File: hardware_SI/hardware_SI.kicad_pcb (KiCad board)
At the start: 2 copper layers, 141.2 x 96.5 mm, 58 parts, among them J1 Barrel_Jack_Switch, J2 Conn_01x07_Female, J3 USB_B_Micro, Q1 SI2323DS-T1, Q2 SI2323DS-T1, SW1 SW_SPDT, U1 OMEGA2+, U2 LTC4085EDEPBF, U3 TPS61200DRC, U4 LD1117S33TR_SOT223, U5 MAX6369, U6 MCP3021, U7 USBLC6-2SC6, U8 CH340N

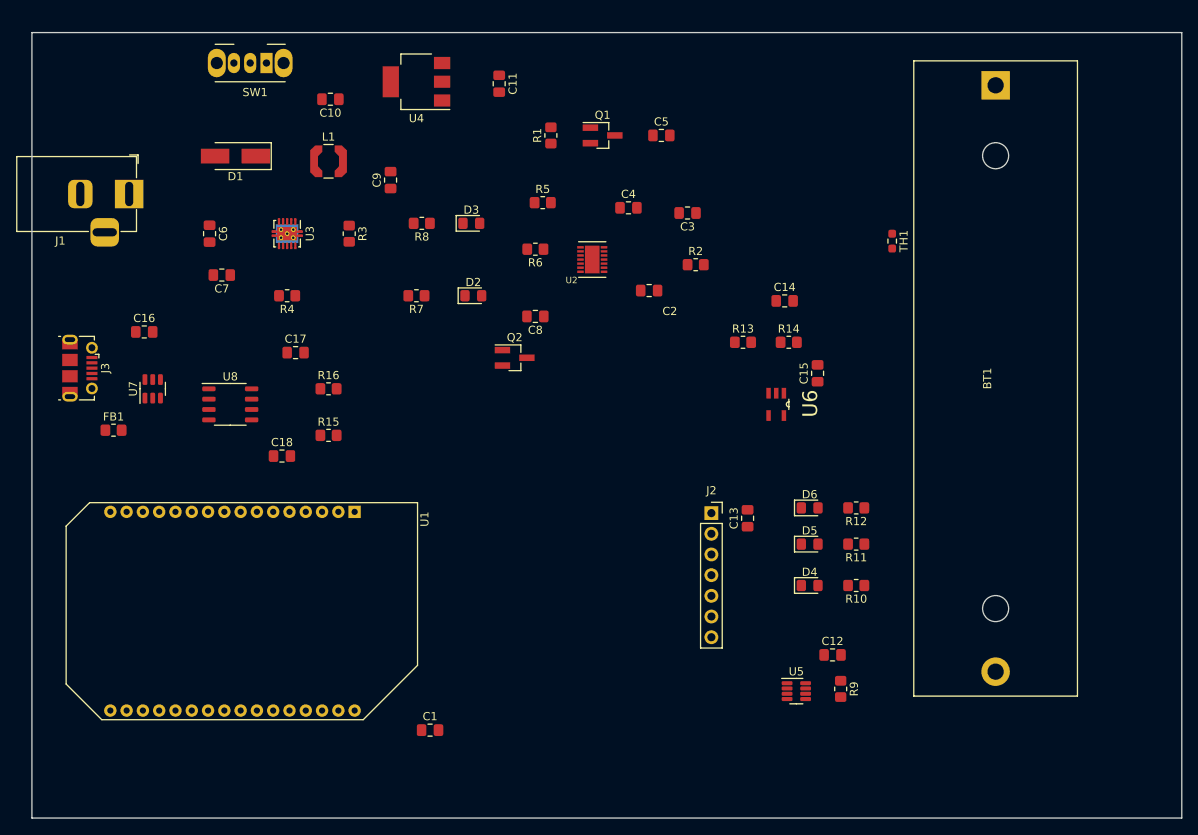
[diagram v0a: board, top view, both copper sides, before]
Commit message: Diseño PCB
No estoy seguro si los huecos de los tornillos se hacen así jaja
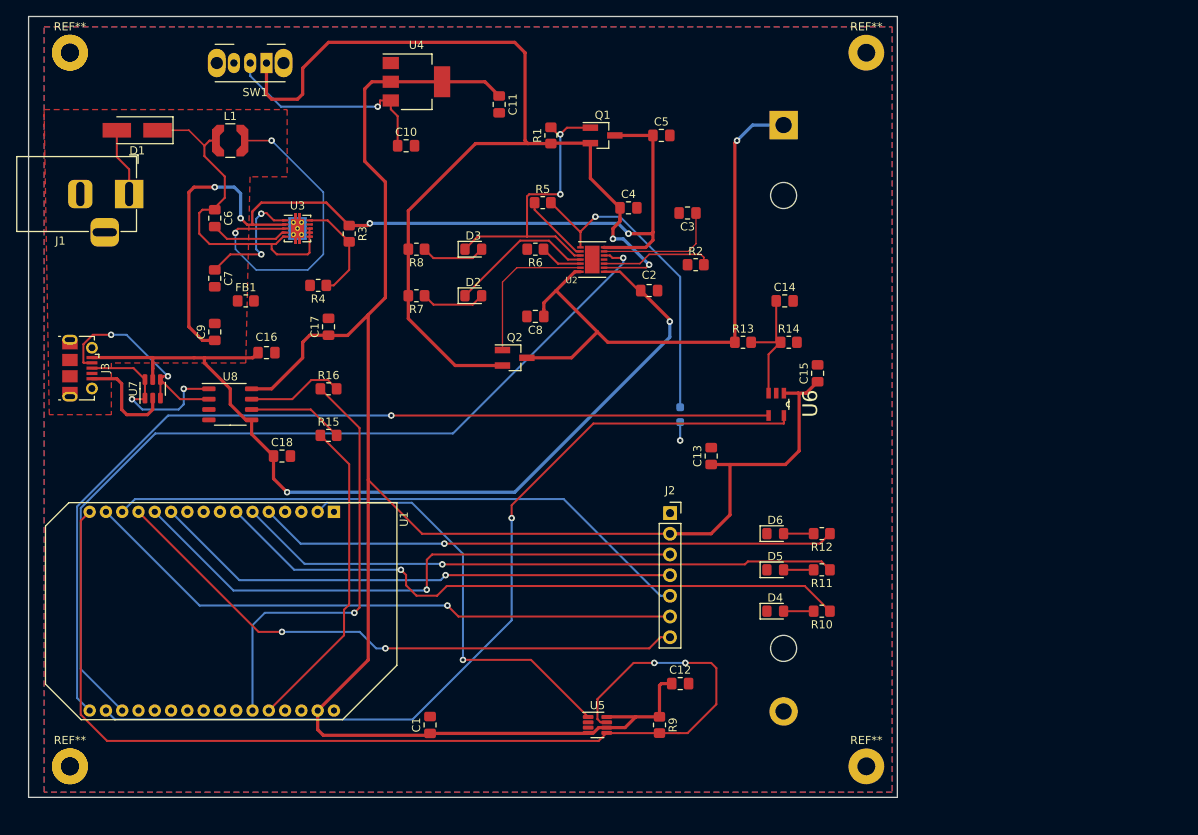
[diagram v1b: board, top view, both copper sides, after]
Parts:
- added ?: , , F.Cu at (52.1, 26.7)
- added ?: , , F.Cu at (52.1, 114.3)
- added REF**: MountingHole_2.2mm_M2_Pad, MountingHole:MountingHole_2.2mm_M2_Pad, F.Cu at (52.1, 114.3)
- added REF**: MountingHole_2.2mm_M2_Pad, MountingHole:MountingHole_2.2mm_M2_Pad, F.Cu at (52.1, 26.7)
- added REF**: MountingHole_2.2mm_M2_Pad, MountingHole:MountingHole_2.2mm_M2_Pad, F.Cu at (149.9, 114.3)
- added REF**: MountingHole_2.2mm_M2_Pad, MountingHole:MountingHole_2.2mm_M2_Pad, F.Cu at (149.9, 26.7)
- BT1, TH1: moved to B.Cu
- moved TH1 33.6 mm to (127.0, 71.1)
- moved C9 28.5 mm to (69.8, 61.0)
- moved BT1 26.5 mm to (139.7, 35.6)
- moved U5 24.8 mm to (116.8, 109.2)
- moved FB1 22.7 mm to (73.7, 57.1)
- moved R9 22.7 mm to (124.5, 109.2)
- moved C12 19.0 mm to (127.0, 104.1)
- moved C16 15.2 mm to (76.2, 63.5), turned to 180 degrees
- moved D1 12.5 mm to (60.3, 36.2)
- moved L1 12.3 mm to (71.8, 37.5)
- moved C10 10.9 mm to (93.3, 38.1), turned to 0 degrees
- moved C13 8.85 mm to (130.8, 76.2)
- moved R10 5.27 mm to (144.4, 95.2)
- moved R11 5.27 mm to (144.4, 90.2)
- moved R12 5.27 mm to (144.4, 85.7)
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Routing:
- net +3V3: track 0.00 -> 249.9 mm
- net +5VL: track 0.00 -> 132.0 mm, vias 0 -> 2
- net /RST_W: track 0.00 -> 131.8 mm, vias 0 -> 2
- net /SDA: track 0.00 -> 115.2 mm, vias 0 -> 1
- net +5VP: track 0.00 -> 113.5 mm, vias 0 -> 4
- net +5VA: track 0.00 -> 113.1 mm, vias 0 -> 2
- net /IO19: track 0.00 -> 109.2 mm, vias 0 -> 1
- net /SCL: track 0.00 -> 108.0 mm, vias 0 -> 1
- net /IO15: track 0.00 -> 79.7 mm, vias 0 -> 1
- net +BATT: track 0.00 -> 74.9 mm, vias 0 -> 1
- net /D/C: track 0.00 -> 74.6 mm, vias 0 -> 1
- net /IO16: track 0.00 -> 74.1 mm, vias 0 -> 1
- net /RST_OLED: track 0.00 -> 72.8 mm
- net /CS1: track 0.00 -> 72.8 mm, vias 0 -> 2
- net /SPI_CLK: track 0.00 -> 71.3 mm, vias 0 -> 1
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- added copper zone on B.Cu, net GND
- added copper zone on F.Cu, net GND
- added copper zone on F.Cu, net GNDPWR
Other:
- board size 141.2 x 96.5 mm -> 106.7 x 95.9 mm
